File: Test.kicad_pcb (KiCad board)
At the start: 6 copper layers, 81 x 62.5 mm, 1 part, among them U1 LTC2942-1

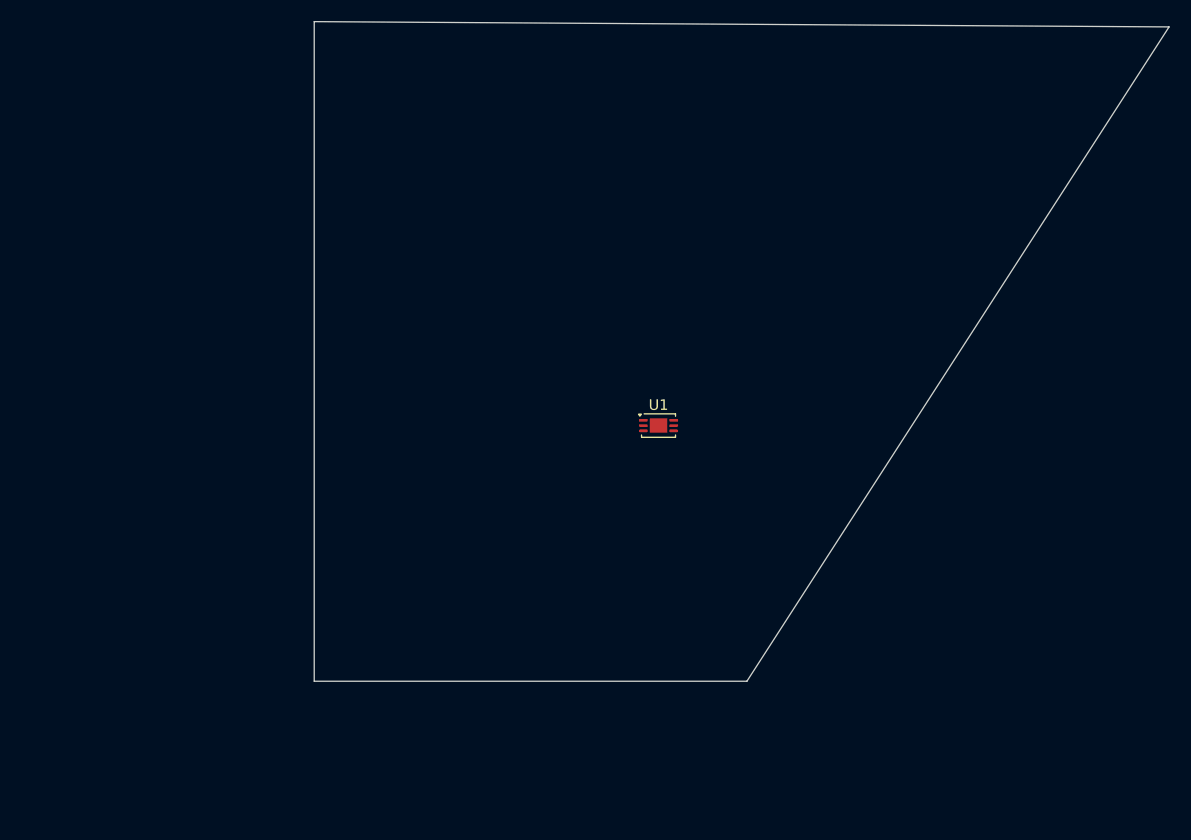
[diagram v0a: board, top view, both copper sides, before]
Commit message: test
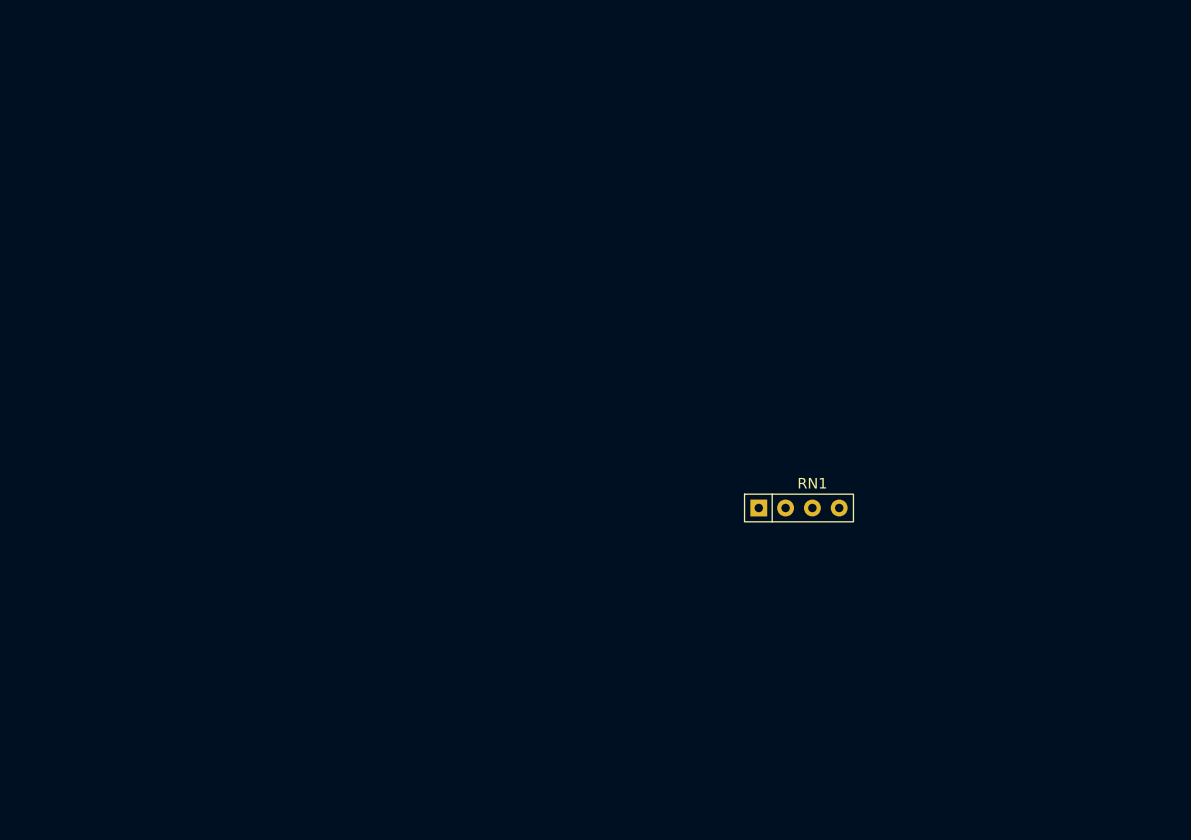
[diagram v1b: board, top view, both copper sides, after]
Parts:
- removed U1: LTC2942-1, Package_DFN_QFN:DFN-6-1EP_3x2mm_P0.5mm_EP1.65x1.35mm
- added RN1: R_Pack02_SIP_Split, Resistor_THT:R_Array_SIP4, F.Cu at (163.6, 100.6)
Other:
- board outline removed
- board text removed: "${FABRICATION_NOTES}"
- board text removed: "3× 120°"

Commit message: test
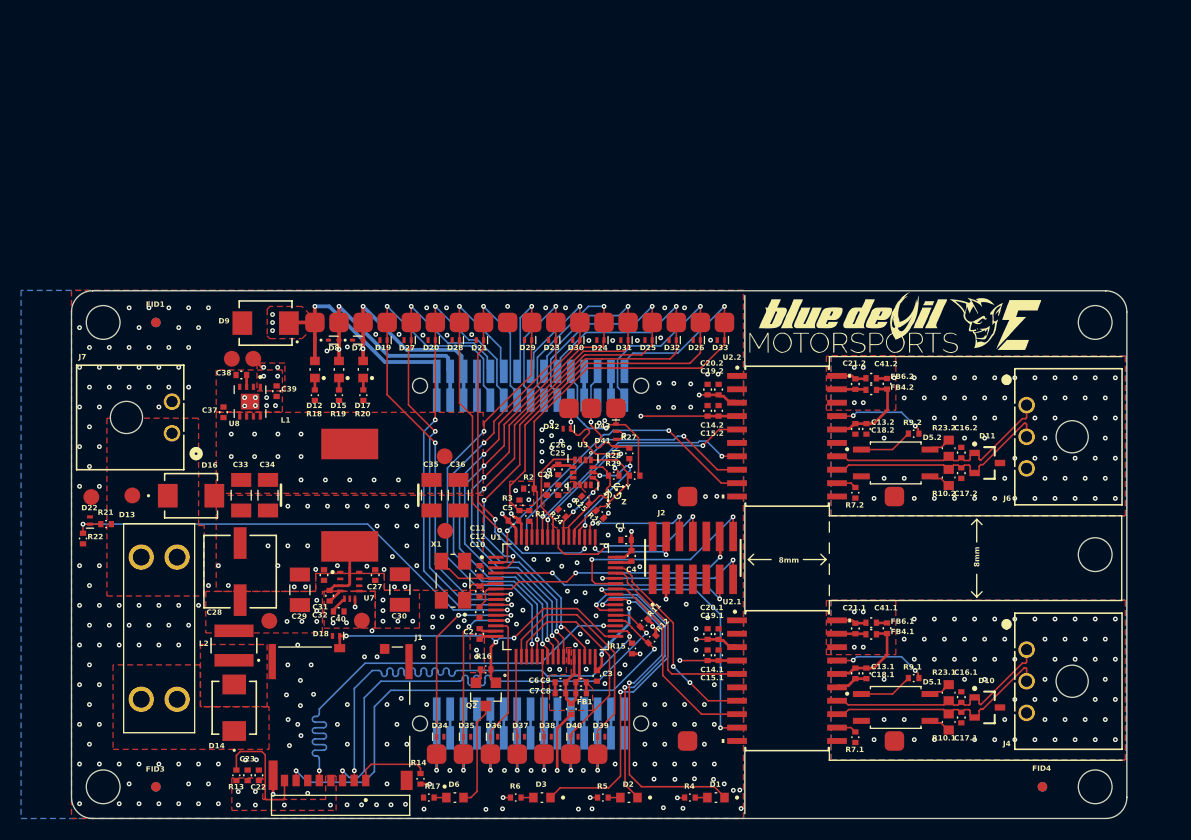
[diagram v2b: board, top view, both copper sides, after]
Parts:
- removed RN1: R_Pack02_SIP_Split, Resistor_THT:R_Array_SIP4
- added ?: , , F.Cu at (101.5, 83.0)
- added ?: , , F.Cu at (101.5, 127.0)
- added ?: , , F.Cu at (195.5, 127.0)
- added ?: , , F.Cu at (195.5, 83.0)
- added ?: , , F.Cu at (195.5, 105.0)
- added C1: 4.7uF, STM32_Telemetry_And_IMU_Module:CL05, F.Cu at (151.1, 103.6)
- added C10: 100nF, STM32_Telemetry_And_IMU_Module:CL05, F.Cu at (137.2, 110.4)
- added C11: 12pF, STM32_Telemetry_And_IMU_Module:CL05, F.Cu at (137.2, 106.5)
- added C12: 12pF, STM32_Telemetry_And_IMU_Module:CL05, F.Cu at (137.2, 108.5)
- added C13.1: 100nF, STM32_Telemetry_And_IMU_Module:CL05, F.Cu at (173.8, 116.3)
- added C13.2: 100nF, STM32_Telemetry_And_IMU_Module:CL05, F.Cu at (173.8, 93.1)
- added C14.1: 10nF, STM32_Telemetry_And_IMU_Module:CL05, F.Cu at (159.8, 114.5)
- added C14.2: 10nF, STM32_Telemetry_And_IMU_Module:CL05, F.Cu at (159.8, 91.4)
- added C15.1: 100nF, STM32_Telemetry_And_IMU_Module:CL05, F.Cu at (158.8, 114.5)
- added C15.2: 100nF, STM32_Telemetry_And_IMU_Module:CL05, F.Cu at (158.8, 91.4)
- added C16.1: 68pF, STM32_Telemetry_And_IMU_Module:CL05, F.Cu at (182.8, 118.5)
- added C16.2: 68pF, STM32_Telemetry_And_IMU_Module:CL05, F.Cu at (182.8, 95.3)
- added C17.1: 68pF, STM32_Telemetry_And_IMU_Module:CL05, F.Cu at (182.8, 120.4)
- added C17.2: 68pF, STM32_Telemetry_And_IMU_Module:CL05, F.Cu at (182.8, 97.3)
- added C18.1: 10nF, STM32_Telemetry_And_IMU_Module:CL05, F.Cu at (172.8, 116.3)
- added C18.2: 10nF, STM32_Telemetry_And_IMU_Module:CL05, F.Cu at (172.8, 93.1)
- added C19.1: 10uF, STM32_Telemetry_And_IMU_Module:CL05, F.Cu at (158.8, 112.5)
- added C19.2: 10uF, STM32_Telemetry_And_IMU_Module:CL05, F.Cu at (158.8, 89.4)
- added C2: 100nF, STM32_Telemetry_And_IMU_Module:CL05, F.Cu at (137.2, 112.5)
- added C20.1: 100nF, STM32_Telemetry_And_IMU_Module:CL05, F.Cu at (159.8, 112.5)
- added C20.2: 100nF, STM32_Telemetry_And_IMU_Module:CL05, F.Cu at (159.8, 89.4)
- added C21.1: 220nF, STM32_Telemetry_And_IMU_Module:CL05, F.Cu at (172.8, 112.0)
- added C21.2: 220nF, STM32_Telemetry_And_IMU_Module:CL05, F.Cu at (172.8, 88.8)
- added C22: 10uF, STM32_Telemetry_And_IMU_Module:CL05, F.Cu at (116.3, 125.9)
- added C23: 100nF, STM32_Telemetry_And_IMU_Module:CL05, F.Cu at (115.2, 125.9)
- added C24: 10uF, STM32_Telemetry_And_IMU_Module:CL05, F.Cu at (143.6, 98.9)
- added C25: 100nF, STM32_Telemetry_And_IMU_Module:CL05, F.Cu at (144.6, 98.9)
- added C26: 100nF, STM32_Telemetry_And_IMU_Module:CL05, F.Cu at (144.6, 96.9)
- added C27: 0.1uF, STM32_Telemetry_And_IMU_Module:CL05, F.Cu at (127.3, 106.9)
- added C28: 47uF, STM32_Telemetry_And_IMU_Module:CAP_UCD_6P3X7P7_NCH, F.Cu at (114.5, 106.6)
- added C29: 4.7uF, STM32_Telemetry_And_IMU_Module:CAPC3216X190N, F.Cu at (120.1, 108.3)
- added C3: 100nF, STM32_Telemetry_And_IMU_Module:CL05, F.Cu at (148.3, 116.5)
- added C30: 4.7uF, STM32_Telemetry_And_IMU_Module:CAPC3216X190N, F.Cu at (129.6, 108.3)
- added C31: 0.1uF, STM32_Telemetry_And_IMU_Module:CL05, F.Cu at (122.4, 106.9)
- added C32: 100nF, STM32_Telemetry_And_IMU_Module:CL05, F.Cu at (123.0, 108.9)
- added C33: 22uF, STM32_Telemetry_And_IMU_Module:CAPC3216X190N, F.Cu at (114.6, 99.4)
- added C34: 22uF, STM32_Telemetry_And_IMU_Module:CAPC3216X190N, F.Cu at (117.1, 99.4)
- added C35: 22uF, STM32_Telemetry_And_IMU_Module:CAPC3216X190N, F.Cu at (132.6, 99.4)
- added C36: 22uF, STM32_Telemetry_And_IMU_Module:CAPC3216X190N, F.Cu at (135.2, 99.4)
- added C37: 1uF, STM32_Telemetry_And_IMU_Module:CL05, F.Cu at (112.9, 91.5)
- added C38: 10nF, STM32_Telemetry_And_IMU_Module:CL05, F.Cu at (114.6, 88.0)
- added C39: 10uF, STM32_Telemetry_And_IMU_Module:CL05, F.Cu at (117.9, 89.5)
- added C4: 100nF, STM32_Telemetry_And_IMU_Module:CL05, F.Cu at (151.6, 105.1)
- added C40: 1uF, STM32_Telemetry_And_IMU_Module:CL05, F.Cu at (123.8, 110.4)
- added C41.1: 10uF, STM32_Telemetry_And_IMU_Module:CL05, F.Cu at (175.8, 112.0)
- added C41.2: 10uF, STM32_Telemetry_And_IMU_Module:CL05, F.Cu at (175.8, 88.8)
- added C5: 100nF, STM32_Telemetry_And_IMU_Module:CL05, F.Cu at (140.4, 101.8)
- added C6: 100nF, STM32_Telemetry_And_IMU_Module:CL05, F.Cu at (144.8, 117.1)
- added C7: 1uF, STM32_Telemetry_And_IMU_Module:CL05, F.Cu at (144.8, 118.1)
- added C8: 1uF, STM32_Telemetry_And_IMU_Module:CL05, F.Cu at (146.8, 118.1)
- added C9: 10nF, STM32_Telemetry_And_IMU_Module:CL05, F.Cu at (146.8, 117.1)
- added D1: LTST-C190TBKT, STM32_Telemetry_And_IMU_Module:LEDC1608X35N, F.Cu at (159.6, 128.0)
- added D10: PESD2CANFD24LT-QR, STM32_Telemetry_And_IMU_Module:SOT95P245X110-3N, F.Cu at (185.3, 119.5)
- added D11: PESD2CANFD24LT-QR, STM32_Telemetry_And_IMU_Module:SOT95P245X110-3N, F.Cu at (185.3, 96.3)
- added D12: LTST-C190KGKT, STM32_Telemetry_And_IMU_Module:LEDC1608X35N, F.Cu at (121.6, 87.5)
- added D13: 3557-2, STM32_Telemetry_And_IMU_Module:FUSE_3557-2, F.Cu at (106.8, 112.0)
- added D14: CDBA340L-HF, STM32_Telemetry_And_IMU_Module:DO-214AASMB_J-BEND_LTF, F.Cu at (113.9, 119.5)
- added D15: LTST-C190KGKT, STM32_Telemetry_And_IMU_Module:LEDC1608X35N, F.Cu at (123.8, 87.5)
- added D16: SMBJ15A, STM32_Telemetry_And_IMU_Module:DO-214AASMB_J-BEND_LTF, F.Cu at (109.8, 99.4)
- added D17: LTST-C190KGKT, STM32_Telemetry_And_IMU_Module:LEDC1608X35N, F.Cu at (126.1, 87.5)
- added D18: TPD1E04U04DPYR, STM32_Telemetry_And_IMU_Module:DPY2_TEX, F.Cu at (123.6, 112.7)
- added D19: TPD1E04U04DPYR, STM32_Telemetry_And_IMU_Module:DPY2_TEX, F.Cu at (128.1, 84.7)
- added D2: LTST-C190TBKT, STM32_Telemetry_And_IMU_Module:LEDC1608X35N, F.Cu at (151.3, 128.0)
- added D20: TPD1E04U04DPYR, STM32_Telemetry_And_IMU_Module:DPY2_TEX, F.Cu at (132.6, 84.7)
- added D21: TPD1E04U04DPYR, STM32_Telemetry_And_IMU_Module:DPY2_TEX, F.Cu at (137.2, 84.7)
- added D22: TPD1E04U04DPYR, STM32_Telemetry_And_IMU_Module:DPY2_TEX, F.Cu at (100.3, 101.8)
- added D23: TPD1E04U04DPYR, STM32_Telemetry_And_IMU_Module:DPY2_TEX, F.Cu at (144.1, 84.7)
- added D24: TPD1E04U04DPYR, STM32_Telemetry_And_IMU_Module:DPY2_TEX, F.Cu at (148.6, 84.7)
- added D25: TPD1E04U04DPYR, STM32_Telemetry_And_IMU_Module:DPY2_TEX, F.Cu at (153.2, 84.7)
- added D26: TPD1E04U04DPYR, STM32_Telemetry_And_IMU_Module:DPY2_TEX, F.Cu at (157.7, 84.7)
- added D27: TPD1E04U04DPYR, STM32_Telemetry_And_IMU_Module:DPY2_TEX, F.Cu at (130.4, 84.7)
- added D28: TPD1E04U04DPYR, STM32_Telemetry_And_IMU_Module:DPY2_TEX, F.Cu at (134.9, 84.7)
- added D29: TPD1E04U04DPYR, STM32_Telemetry_And_IMU_Module:DPY2_TEX, F.Cu at (141.8, 84.7)
- added D3: LTST-C190TBKT, STM32_Telemetry_And_IMU_Module:LEDC1608X35N, F.Cu at (143.1, 128.0)
- added D30: TPD1E04U04DPYR, STM32_Telemetry_And_IMU_Module:DPY2_TEX, F.Cu at (146.3, 84.7)
- added D31: TPD1E04U04DPYR, STM32_Telemetry_And_IMU_Module:DPY2_TEX, F.Cu at (150.9, 84.7)
- added D32: TPD1E04U04DPYR, STM32_Telemetry_And_IMU_Module:DPY2_TEX, F.Cu at (155.5, 84.7)
- added D33: TPD1E04U04DPYR, STM32_Telemetry_And_IMU_Module:DPY2_TEX, F.Cu at (160.0, 84.7)
- added D34: TPD1E04U04DPYR, STM32_Telemetry_And_IMU_Module:DPY2_TEX, F.Cu at (133.4, 122.3)
- added D35: TPD1E04U04DPYR, STM32_Telemetry_And_IMU_Module:DPY2_TEX, F.Cu at (136.0, 122.3)
- added D36: TPD1E04U04DPYR, STM32_Telemetry_And_IMU_Module:DPY2_TEX, F.Cu at (138.5, 122.3)
- added D37: TPD1E04U04DPYR, STM32_Telemetry_And_IMU_Module:DPY2_TEX, F.Cu at (141.1, 122.3)
- added D38: TPD1E04U04DPYR, STM32_Telemetry_And_IMU_Module:DPY2_TEX, F.Cu at (143.6, 122.3)
- added D39: TPD1E04U04DPYR, STM32_Telemetry_And_IMU_Module:DPY2_TEX, F.Cu at (148.7, 122.3)
- added D40: TPD1E04U04DPYR, STM32_Telemetry_And_IMU_Module:DPY2_TEX, F.Cu at (146.2, 122.3)
- added D41: TPD1E04U04DPYR, STM32_Telemetry_And_IMU_Module:DPY2_TEX, F.Cu at (150.1, 94.4)
- added D42: TPD1E04U04DPYR, STM32_Telemetry_And_IMU_Module:DPY2_TEX, F.Cu at (145.4, 93.1)
- added D43: TPD1E04U04DPYR, STM32_Telemetry_And_IMU_Module:DPY2_TEX, F.Cu at (150.1, 93.0)
- added D5.1: TLP172AM(TPR,E, STM32_Telemetry_And_IMU_Module:SOIC254P700X220-4N, F.Cu at (176.6, 119.5)
- added D5.2: TLP172AM(TPR,E, STM32_Telemetry_And_IMU_Module:SOIC254P700X220-4N, F.Cu at (176.6, 96.3)
- added D6: LTST-C190KGKT, STM32_Telemetry_And_IMU_Module:LEDC1608X35N, F.Cu at (134.8, 128.0)
- added D7: ESD9B3.3ST5G, STM32_Telemetry_And_IMU_Module:SODFL1006X40N, F.Cu at (125.6, 84.7)
- added D8: ESD9B5.0ST5G, STM32_Telemetry_And_IMU_Module:SODFL1006X40N, F.Cu at (123.3, 84.7)
- added D9: CDBA340L-HF, STM32_Telemetry_And_IMU_Module:DO-214AASMB_J-BEND_LTF, F.Cu at (116.9, 83.1)
- added FB1: 330 Ohms @ 100 MHz, STM32_Telemetry_And_IMU_Module:BLM15EX331SN1D, F.Cu at (145.9, 119.6)
- added FB4.1: 330 Ohms @ 100 MHz, STM32_Telemetry_And_IMU_Module:BLM15EX331SN1D, F.Cu at (174.3, 112.6)
- added FB4.2: 330 Ohms @ 100 MHz, STM32_Telemetry_And_IMU_Module:BLM15EX331SN1D, F.Cu at (174.3, 89.4)
- added FB6.1: 330 Ohms @ 100 MHz, STM32_Telemetry_And_IMU_Module:BLM15EX331SN1D, F.Cu at (174.3, 111.5)
- added FB6.2: 330 Ohms @ 100 MHz, STM32_Telemetry_And_IMU_Module:BLM15EX331SN1D, F.Cu at (174.3, 88.3)
- added FID1: DNP, STM32_Telemetry_And_IMU_Module:FID90X190, F.Cu at (106.5, 83.0)
- added FID2: DNP, STM32_Telemetry_And_IMU_Module:FID90X190, B.Cu at (190.5, 127.0)
- added FID3: DNP, STM32_Telemetry_And_IMU_Module:FID90X190, F.Cu at (106.5, 127.0)
- added FID4: DNP, STM32_Telemetry_And_IMU_Module:FID90X190, F.Cu at (190.5, 127.0)
- added FID5: DNP, STM32_Telemetry_And_IMU_Module:FID90X190, B.Cu at (106.5, 83.0)
- added FID6: DNP, STM32_Telemetry_And_IMU_Module:FID90X190, B.Cu at (106.5, 127.0)
- added J1: 503398-1892, STM32_Telemetry_And_IMU_Module:MOLEX_503398-1892, F.Cu at (124.0, 120.8)
- added J2: FTSH-107-01-L-DV-K-TR, STM32_Telemetry_And_IMU_Module:SAMTEC_FTSH-107-01-X-DV-K-TR, F.Cu at (157.4, 105.3)
- added J3: SFM-115-02-L-D-A-K-TR, STM32_Telemetry_And_IMU_Module:SAMTEC_SFM-115-02-X-D-A, B.Cu at (142.0, 89.0)
- added J4: 0436500300, STM32_Telemetry_And_IMU_Module:CONN_SD-43650-001_03_MOL, F.Cu at (189.0, 114.0)
- added J5: SFM-115-02-L-D-A-K-TR, STM32_Telemetry_And_IMU_Module:SAMTEC_SFM-115-02-X-D-A, B.Cu at (142.0, 121.0)
- added J6: 0436500300, STM32_Telemetry_And_IMU_Module:CONN_SD-43650-001_03_MOL, F.Cu at (189.0, 90.8)
- added J7: 0436500200, STM32_Telemetry_And_IMU_Module:CONN_SD-43650-001_02_MOL, F.Cu at (108.0, 93.5)
- added L1: 10 µH, STM32_Telemetry_And_IMU_Module:PM124SH-100M-RC, F.Cu at (124.9, 99.4)
- added L2: 2.2uH, STM32_Telemetry_And_IMU_Module:IND_TAIYO_NRS4018_TAY, F.Cu at (113.9, 113.6)
- added Q2: BSS84, STM32_Telemetry_And_IMU_Module:SOT95P240X120-3N, F.Cu at (137.8, 118.2)
- added R1: 0, STM32_Telemetry_And_IMU_Module:RMCF0402FT, F.Cu at (141.9, 101.3)
- added R10.1: 59R, STM32_Telemetry_And_IMU_Module:RESC1508X50N, F.Cu at (181.6, 118.1)
- added R10.2: 59R, STM32_Telemetry_And_IMU_Module:RESC1508X50N, F.Cu at (181.6, 94.9)
- added R11: 10K, STM32_Telemetry_And_IMU_Module:RMCF0402FT, F.Cu at (152.8, 111.5)
- added R12: 10K, STM32_Telemetry_And_IMU_Module:RMCF0402FT, F.Cu at (153.5, 113.0)
- added R13: 10K, STM32_Telemetry_And_IMU_Module:RMCF0402FT, F.Cu at (114.1, 125.9)
- added R14: 10K, STM32_Telemetry_And_IMU_Module:RMCF0402FT, F.Cu at (131.6, 126.2)
- added R15: 10K, STM32_Telemetry_And_IMU_Module:RMCF0402FT, F.Cu at (151.6, 113.9)
- added R16: 10K, STM32_Telemetry_And_IMU_Module:RMCF0402FT, F.Cu at (137.7, 115.9)
- added R17: 240, STM32_Telemetry_And_IMU_Module:RMCF0402FT, F.Cu at (132.4, 128.0)
- added R18: 2k, STM32_Telemetry_And_IMU_Module:RMCF0402FT, F.Cu at (121.6, 89.9)
- added R19: 560R, STM32_Telemetry_And_IMU_Module:RMCF0402FT, F.Cu at (123.8, 89.9)
- added R2: 2k, STM32_Telemetry_And_IMU_Module:RMCF0402FT, F.Cu at (141.8, 98.8)
- added R20: 240, STM32_Telemetry_And_IMU_Module:RMCF0402FT, F.Cu at (126.2, 89.9)
- added R21: 120K, STM32_Telemetry_And_IMU_Module:RMCF0402FT, F.Cu at (101.8, 102.1)
- added R22: 10k, STM32_Telemetry_And_IMU_Module:RMCF0402FT, F.Cu at (99.6, 103.5)
- added R23.1: 59R, STM32_Telemetry_And_IMU_Module:RESC1508X50N, F.Cu at (181.6, 120.9)
- added R23.2: 59R, STM32_Telemetry_And_IMU_Module:RESC1508X50N, F.Cu at (181.6, 97.7)
- added R24: 10K, STM32_Telemetry_And_IMU_Module:RMCF0402FT, F.Cu at (145.0, 101.1)
- added R25: 10K, STM32_Telemetry_And_IMU_Module:RMCF0402FT, F.Cu at (147.2, 99.8)
- added R26: 10K, STM32_Telemetry_And_IMU_Module:RMCF0402FT, F.Cu at (148.6, 101.2)
- added R27: 0, STM32_Telemetry_And_IMU_Module:RMCF0402FT, F.Cu at (151.4, 95.4)
- added R28: 0, STM32_Telemetry_And_IMU_Module:RMCF0402FT, F.Cu at (149.9, 97.5)
- added R29: 0, STM32_Telemetry_And_IMU_Module:RMCF0402FT, F.Cu at (151.9, 97.5)
- added R3: 2k, STM32_Telemetry_And_IMU_Module:RMCF0402FT, F.Cu at (140.9, 100.3)
- added R4: 240, STM32_Telemetry_And_IMU_Module:RMCF0402FT, F.Cu at (157.1, 128.0)
- added R5: 240, STM32_Telemetry_And_IMU_Module:RMCF0402FT, F.Cu at (148.9, 128.0)
- added R6: 240, STM32_Telemetry_And_IMU_Module:RMCF0402FT, F.Cu at (140.6, 128.0)
- added R7.1: 0, STM32_Telemetry_And_IMU_Module:RMCF0402FT, F.Cu at (172.8, 122.3)
- added R7.2: 0, STM32_Telemetry_And_IMU_Module:RMCF0402FT, F.Cu at (172.8, 99.1)
- added R9.1: 240, STM32_Telemetry_And_IMU_Module:RMCF0402FT, F.Cu at (178.3, 116.7)
- added R9.2: 240, STM32_Telemetry_And_IMU_Module:RMCF0402FT, F.Cu at (178.3, 93.5)
- added TP1: NA, STM32_Telemetry_And_IMU_Module:TP150-NO3D, F.Cu at (117.2, 111.3)
- added TP10: TP-Square, STM32_Telemetry_And_IMU_Module:TPS180, F.Cu at (126.1, 83.0)
- added TP11: TP-Square, STM32_Telemetry_And_IMU_Module:TPS180, F.Cu at (123.8, 83.0)
- added TP12: TP-Square, STM32_Telemetry_And_IMU_Module:TPS180, F.Cu at (121.6, 83.0)
- added TP13: TP-Square, STM32_Telemetry_And_IMU_Module:TPS180, F.Cu at (128.4, 83.0)
- added TP14: TP-Square, STM32_Telemetry_And_IMU_Module:TPS180, F.Cu at (133.0, 83.0)
- added TP15: TP-Square, STM32_Telemetry_And_IMU_Module:TPS180, F.Cu at (137.5, 83.0)
- added TP16: TP-Square, STM32_Telemetry_And_IMU_Module:TPS180, F.Cu at (139.8, 83.0)
- added TP17: TP-Square, STM32_Telemetry_And_IMU_Module:TPS180, F.Cu at (144.4, 83.0)
- added TP18: TP-Square, STM32_Telemetry_And_IMU_Module:TPS180, F.Cu at (149.0, 83.0)
- added TP19: TP-Square, STM32_Telemetry_And_IMU_Module:TPS180, F.Cu at (153.5, 83.0)
- added TP2: NA, STM32_Telemetry_And_IMU_Module:TP150-NO3D, F.Cu at (133.9, 95.7)
- added TP20: TP-Square, STM32_Telemetry_And_IMU_Module:TPS180, F.Cu at (158.1, 83.0)
- added TP21: TP-Square, STM32_Telemetry_And_IMU_Module:TPS180, F.Cu at (130.7, 83.0)
- added TP22: TP-Square, STM32_Telemetry_And_IMU_Module:TPS180, F.Cu at (135.3, 83.0)
- added TP23: TP-Square, STM32_Telemetry_And_IMU_Module:TPS180, F.Cu at (142.1, 83.0)
- added TP24: TP-Square, STM32_Telemetry_And_IMU_Module:TPS180, F.Cu at (146.7, 83.0)
- added TP25: TP-Square, STM32_Telemetry_And_IMU_Module:TPS180, F.Cu at (151.2, 83.0)
- added TP26: TP-Square, STM32_Telemetry_And_IMU_Module:TPS180, F.Cu at (155.8, 83.0)
- added TP27: TP-Square, STM32_Telemetry_And_IMU_Module:TPS180, F.Cu at (160.4, 83.0)
- added TP28: TP-Square, STM32_Telemetry_And_IMU_Module:TPS180, F.Cu at (133.1, 123.9)
- added TP29: TP-Square, STM32_Telemetry_And_IMU_Module:TPS180, F.Cu at (135.6, 123.9)
- added TP3: NA, STM32_Telemetry_And_IMU_Module:TP150-NO3D, F.Cu at (115.7, 86.4)
- added TP30: TP-Square, STM32_Telemetry_And_IMU_Module:TPS180, F.Cu at (138.2, 123.9)
- added TP31: TP-Square, STM32_Telemetry_And_IMU_Module:TPS180, F.Cu at (140.7, 123.9)
- added TP32: TP-Square, STM32_Telemetry_And_IMU_Module:TPS180, F.Cu at (143.3, 123.9)
- added TP33: TP-Square, STM32_Telemetry_And_IMU_Module:TPS180, F.Cu at (148.4, 123.9)
- added TP34: TP-Square, STM32_Telemetry_And_IMU_Module:TPS180, F.Cu at (145.8, 123.9)
- added TP35: TP-Square, STM32_Telemetry_And_IMU_Module:TPS180, F.Cu at (176.5, 122.7)
- added TP36: TP-Square, STM32_Telemetry_And_IMU_Module:TPS180, F.Cu at (156.9, 122.7)
- added TP37: TP-Square, STM32_Telemetry_And_IMU_Module:TPS180, F.Cu at (176.5, 99.5)
- added TP38: NA, STM32_Telemetry_And_IMU_Module:TP150-NO3D, F.Cu at (100.4, 99.5)
- added TP39: TP-Square, STM32_Telemetry_And_IMU_Module:TPS180, F.Cu at (145.6, 91.1)
- added TP4: NA, STM32_Telemetry_And_IMU_Module:TP150-NO3D, F.Cu at (133.9, 102.7)
- added TP40: TP-Square, STM32_Telemetry_And_IMU_Module:TPS180, F.Cu at (150.1, 91.1)
- added TP5: NA, STM32_Telemetry_And_IMU_Module:TP150-NO3D, F.Cu at (126.0, 111.3)
- added TP6: NA, STM32_Telemetry_And_IMU_Module:TP150-NO3D, F.Cu at (113.7, 86.4)
- added TP7: NA, STM32_Telemetry_And_IMU_Module:TP150-NO3D, F.Cu at (104.3, 99.4)
- added TP8: TP-Square, STM32_Telemetry_And_IMU_Module:TPS180, F.Cu at (147.8, 91.1)
- added TP9: TP-Square, STM32_Telemetry_And_IMU_Module:TPS180, F.Cu at (156.9, 99.5)
- added U1: STM32G474RCT6, STM32_Telemetry_And_IMU_Module:QFP50P1200X1200X160-64N, F.Cu at (144.4, 109.0)
- added U2.1: ADM3057EBRWZ, STM32_Telemetry_And_IMU_Module:RW-20_ADI, F.Cu at (166.3, 116.9)
- added U2.2: ADM3057EBRWZ, STM32_Telemetry_And_IMU_Module:RW-20_ADI, F.Cu at (166.3, 93.8)
- added U3: ASM330LHHG1TR, STM32_Telemetry_And_IMU_Module:LGA14_2P5X3_STM, F.Cu at (147.0, 97.2)
- added U7: LMR33620AQ5RNXTQ1, STM32_Telemetry_And_IMU_Module:RNX0012B, F.Cu at (124.9, 107.8)
- added U8: TPS73733QDRBRQ1, STM32_Telemetry_And_IMU_Module:IC_DRV8601DRBT, F.Cu at (115.4, 90.5)
- added X1: 8Mhz, STM32_Telemetry_And_IMU_Module:XTAL_ECS-80-10-30B-CWN-TR, F.Cu at (134.7, 107.5)
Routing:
- net 3V3: track 0.00 -> 74.3 mm, vias 0 -> 34
- net GPIO_6: track 0.00 -> 63.4 mm, vias 0 -> 3
- net GPIO_5: track 0.00 -> 57.2 mm, vias 0 -> 3
- net GPIO_4: track 0.00 -> 57.2 mm, vias 0 -> 3
- net GPIO_7: track 0.00 -> 54.3 mm, vias 0 -> 3
- net GPIO_2: track 0.00 -> 52.7 mm, vias 0 -> 3
- net TIM1_CH1: track 0.00 -> 51.5 mm, vias 0 -> 3
- net GPIO_3: track 0.00 -> 51.0 mm, vias 0 -> 3
- net SD_MISO: track 0.00 -> 49.0 mm, vias 0 -> 2
- net TIM1_CH3: track 0.00 -> 48.7 mm, vias 0 -> 3
- net GPIO_1: track 0.00 -> 48.6 mm, vias 0 -> 3
- net I2C1_SDA: track 0.00 -> 48.5 mm, vias 0 -> 1
- net I2C1_SCL: track 0.00 -> 48.2 mm, vias 0 -> 1
- net TIM2_CH3: track 0.00 -> 48.0 mm, vias 0 -> 3
- net VBAT_ADC: track 0.00 -> 47.2 mm, vias 0 -> 2
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- added copper zone on F.Cu, net 12V
- added copper zone on In2.Cu, net 12V
- added copper zone on F.Cu, net 3V3
- added copper zone on In2.Cu, net 3V3
- added copper zone on F.Cu, net 5V
- added copper zone on In2.Cu, net 5V
- added copper zone on B.Cu, net GND
- added copper zone on F.Cu, net GND
- added copper zone on In1.Cu, net GND
- added copper zone on In2.Cu, net GND
- added copper zone on F.Cu, net GNDISO.1
- added copper zone on In1.Cu, net GNDISO.1
- added copper zone on F.Cu, net GNDISO.2
- added copper zone on In1.Cu, net GNDISO.2
- added copper zone on B.Cu, net ISO_GND.1
- added copper zone on F.Cu, net ISO_GND.1
- added copper zone on In1.Cu, net ISO_GND.1
- added copper zone on In2.Cu, net ISO_GND.1
- added copper zone on B.Cu, net ISO_GND.2
- added copper zone on F.Cu, net ISO_GND.2
- added copper zone on In1.Cu, net ISO_GND.2
- added copper zone on In2.Cu, net ISO_GND.2
- added copper zone on F.Cu, net NetD13_2_1
- added copper zone on F.Cu, net NetD14_2
- added copper zone on F.Cu, net VBAT
- added copper zone on F.Cu, net VSSA
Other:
- board outline added: 100 x 50 mm
- copper layers 6 -> 4
- rule pad_to_mask_clearance: 0.05 -> 0
- board text added: "8mm"
- board text added: "T.I.M."
- board text added: "Z"
